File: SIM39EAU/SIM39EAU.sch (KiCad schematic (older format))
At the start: 15 parts, among them IC1 SIM39EA, J1 Conn_01x08, U2 AP7365-W-7

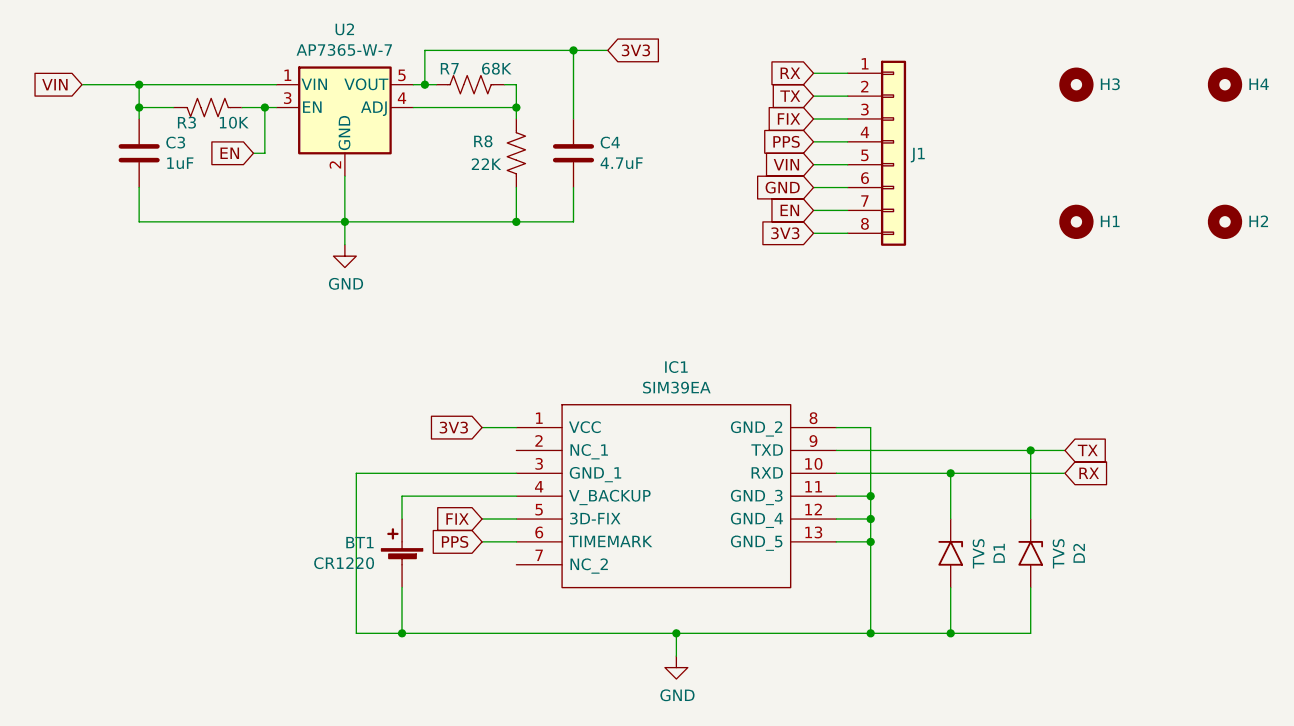
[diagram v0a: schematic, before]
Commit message: LED Update
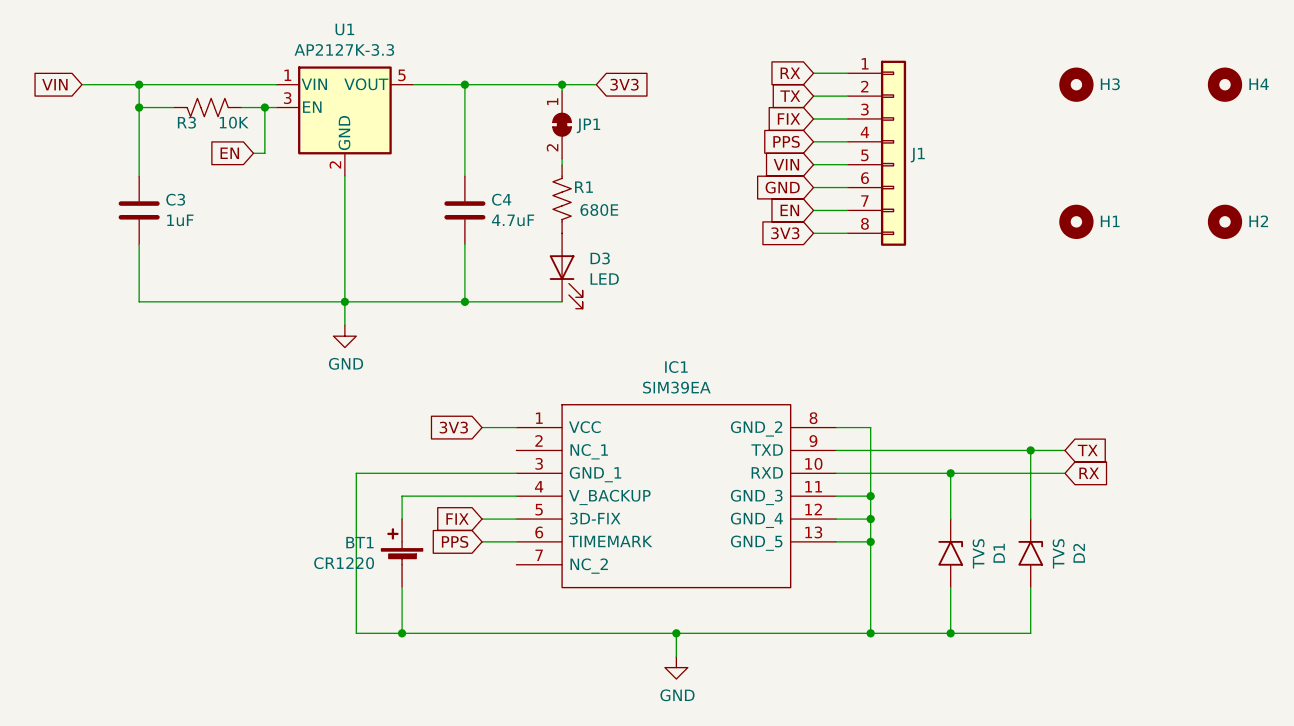
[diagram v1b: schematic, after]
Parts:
- removed R7: 68K, Resistor_SMD:R_0603_1608Metric, symbol Device:R_US
- removed R8: 22K, Resistor_SMD:R_0603_1608Metric, symbol Device:R_US
- removed U2: AP7365-W-7, Package_TO_SOT_SMD:SOT-23-5, symbol Regulator_Linear:AP2127K-ADJ
- added D3: LED, LED_SMD:LED_0603_1608Metric, symbol Device:LED
- added JP1: SolderJumper_2_Bridged, Jumper:SolderJumper-2_P1.3mm_Bridged_RoundedPad1.0x1.5mm, symbol Jumper:SolderJumper_2_Bridged
- added R1: 680E, Resistor_SMD:R_0603_1608Metric, symbol Device:R_US
- added U1: AP2127K-3.3, Package_TO_SOT_SMD:SOT-23-5, symbol Regulator_Linear:AP2127K-3.3
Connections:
- net 3V3: now also JP1.1 (A), U1.5 (VOUT)
- net EN: now also U1.3 (EN)
- net GND: now also D3.1 (K), U1.2 (GND)
- net VIN: now also U1.1 (VIN)
- new net: JP1.2 (B), R1.2
- new net: D3.2 (A), R1.1
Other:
- moved on the sheet: C3, C4
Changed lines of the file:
@@
 Comment4 ""
 $EndDescr
-Text GLabel 3600 1100 2    50   Input ~ 0
+Text GLabel 3550 1250 2    50   Input ~ 0
 3V3
 Wire Wire Line
-	1550 1400 1550 1350
-Wire Wire Line
-	1550 1700 1550 1850
+	1550 1650 1550 1350
+Wire Wire Line
+	1550 1950 1550 2200
 $Comp
 L power:GND #PWR0103
 U 1 1 5DFA7870
-P 2450 1950
-F 0 "#PWR0103" H 2450 1700 50  0001 C CNN
-F 1 "GND" H 2455 1777 50  0000 C CNN
-F 2 "" H 2450 1950 50  0001 C CNN
-F 3 "" H 2450 1950 50  0001 C CNN
-	1    2450 1950
-	1    0    0    -1
-$EndComp
-$Comp
-L Regulator_Linear:AP2127K-ADJ U2
-U 1 1 5E2BA0AD
-P 2450 1350
-F 0 "U2" H 2450 1690 50  0000 C CNN
-F 1 "AP7365-W-7" H 2450 1600 50  0000 C CNN
-F 2 "Package_TO_SOT_SMD:SOT-23-5" H 2450 1675 50  0001 C CNN
-F 3 "https://www.diodes.com/assets/Datasheets/AP2127.pdf" H 2450 1450 50  0001 C CNN
-	1    2450 1350
-	1    0    0    -1
-$EndComp
-$Comp
-L Device:R_US R7
-U 1 1 5E34715F
-P 3000 1250
-F 0 "R7" V 3068 1296 50  0000 L CNN
-F 1 "68K" V 3068 1205 50  0000 R CNN
-F 2 "Resistor_SMD:R_0603_1608Metric" V 3040 1240 50  0001 C CNN
-F 3 "~" H 3000 1250 50  0001 C CNN
-F 4 "C163436" V 3000 1250 50  0001 C CNN "Part"
-	1    3000 1250
-	0    -1   -1   0
-$EndComp
-$Comp
-L Device:R_US R8
-U 1 1 5E35753D
-P 3200 1550
-F 0 "R8" H 3300 1500 50  0000 L CNN
-F 1 "22K" H 3400 1600 50  0000 R CNN
-F 2 "Resistor_SMD:R_0603_1608Metric" V 3240 1540 50  0001 C CNN
-F 3 "~" H 3200 1550 50  0001 C CNN
-F 4 "C103426" H 3200 1550 50  0001 C CNN "Part"
-	1    3200 1550
-	-1   0    0    1
-$EndComp
-Wire Wire Line
-	3200 1350 2750 1350
-Wire Wire Line
-	3150 1250 3200 1250
-Wire Wire Line
-	3200 1400 3200 1350
+P 2450 2300
+F 0 "#PWR0103" H 2450 2050 50  0001 C CNN
+F 1 "GND" H 2455 2127 50  0000 C CNN
+F 2 "" H 2450 2300 50  0001 C CNN
+F 3 "" H 2450 2300 50  0001 C CNN
+	1    2450 2300
+	1    0    0    -1
+$EndComp
 Text GLabel 4500 1300 0    50   Input ~ 0
 TX
@@
 FIX
 Wire Wire Line
-	1550 1850 2450 1850
-Wire Wire Line
-	3200 1700 3200 1850
-Wire Wire Line
-	3200 1350 3200 1250
-Connection ~ 3200 1350
-Wire Wire Line
-	2750 1250 2800 1250
-Wire Wire Line
-	2800 1250 2800 1100
-Connection ~ 2800 1250
-Wire Wire Line
-	2800 1250 2850 1250
-Wire Wire Line
-	2800 1100 3450 1100
+	1550 2200 2450 2200
 $Comp
 L Device:C C3
 U 1 1 5DCB3070
-P 1550 1550
-F 0 "C3" H 1665 1595 50  0000 L CNN
-F 1 "1uF" H 1665 1505 50  0000 L CNN
-F 2 "Capacitor_SMD:C_0805_2012Metric" H 1588 1400 50  0001 C CNN
-F 3 "~" H 1550 1550 50  0001 C CNN
-F 4 "C396719" H 1550 1550 50  0001 C CNN "Part"
-	1    1550 1550
-	1    0    0    -1
-$EndComp
-Wire Wire Line
-	3450 1400 3450 1100
-Connection ~ 3450 1100
-Wire Wire Line
-	3450 1100 3600 1100
-Wire Wire Line
-	3450 1700 3450 1850
-Wire Wire Line
-	3450 1850 3200 1850
-Connection ~ 3200 1850
+P 1550 1800
+F 0 "C3" H 1665 1845 50  0000 L CNN
+F 1 "1uF" H 1665 1755 50  0000 L CNN
+F 2 "Capacitor_SMD:C_0805_2012Metric" H 1588 1650 50  0001 C CNN
+F 3 "~" H 1550 1800 50  0001 C CNN
+F 4 "C396719" H 1550 1800 50  0001 C CNN "Part"
+	1    1550 1800
+	1    0    0    -1
+$EndComp
+Wire Wire Line
+	2975 1950 2975 2200
 Text GLabel 1300 1250 0    50   Input ~ 0
 VIN
@@
 L Device:C C4
 U 1 1 5DB8E885
-P 3450 1550
-F 0 "C4" H 3565 1595 50  0000 L CNN
-F 1 "4.7uF" H 3565 1505 50  0000 L CNN
-F 2 "Capacitor_SMD:C_0805_2012Metric" H 3488 1400 50  0001 C CNN
-F 3 "~" H 3450 1550 50  0001 C CNN
-F 4 "C87998" H 3450 1550 50  0001 C CNN "Part"
-	1    3450 1550
+P 2975 1800
+F 0 "C4" H 3090 1845 50  0000 L CNN
+F 1 "4.7uF" H 3090 1755 50  0000 L CNN
+F 2 "Capacitor_SMD:C_0805_2012Metric" H 3013 1650 50  0001 C CNN
+F 3 "~" H 2975 1800 50  0001 C CNN
+F 4 "C87998" H 2975 1800 50  0001 C CNN "Part"
+	1    2975 1800
 	1    0    0    -1
 $EndComp
@@
 	1    0    0    -1
 $EndComp
-Wire Wire Line
-	2450 1650 2450 1850
-Connection ~ 2450 1850
-Wire Wire Line
-	2450 1850 3200 1850
-Wire Wire Line
-	2450 1850 2450 1950
+Connection ~ 2450 2200
+Wire Wire Line
+	2450 2200 2450 2300
 Wire Wire Line
 	4650 1500 4500 1500
@@
 Wire Wire Line
 	5100 3450 5100 3650
+Wire Wire Line
+	2450 2200 2975 2200
+Wire Wire Line
+	2750 1250 2975 1250
+$Comp
+L Regulator_Linear:AP2127K-3.3 U1
+U 1 1 5DFE50D8
+P 2450 1350
+F 0 "U1" H 2450 1690 50  0000 C CNN
+F 1 "AP2127K-3.3" H 2450 1600 50  0000 C CNN
+F 2 "Package_TO_SOT_SMD:SOT-23-5" H 2450 1675 50  0001 C CNN
+F 3 "https://www.diodes.com/assets/Datasheets/AP2127.pdf" H 2450 1450 50  0001 C CNN
+	1    2450 1350
+	1    0    0    -1
+$EndComp
+Wire Wire Line
+	2975 1650 2975 1250
+Wire Wire Line
+	2450 1650 2450 2200
+Connection ~ 2975 1250
+Connection ~ 2975 2200
+Wire Wire Line
+	2975 1250 3400 1250
+$Comp
+L Jumper:SolderJumper_2_Bridged JP1
+U 1 1 5DFFCA44
+P 3400 1425
+F 0 "JP1" V 3400 1493 50  0000 L CNN
+F 1 "SolderJumper_2_Bridged" V 3445 1493 50  0001 L CNN
+F 2 "Jumper:SolderJumper-2_P1.3mm_Bridged_RoundedPad1.0x1.5mm" H 3400 1425 50  0001 C CNN
+F 3 "~" H 3400 1425 50  0001 C CNN
+	1    3400 1425
+	0    1    1    0
+$EndComp
+$Comp
+L Device:LED D3
+U 1 1 5DFFF072
+P 3400 2050
+F 0 "D3" V 3438 1932 50  0000 R CNN
+F 1 "LED" V 3348 1932 50  0000 R CNN
+F 2 "LED_SMD:LED_0603_1608Metric" H 3400 2050 50  0001 C CNN
+F 3 "~" H 3400 2050 50  0001 C CNN
+F 4 "C193191" V 3400 2050 50  0001 C CNN "Part"
+	1    3400 2050
+	0    -1   -1   0
+$EndComp
+$Comp
+L Device:R_US R1
+U 1 1 5E000844
+P 3400 1750
+F 0 "R1" H 3450 1700 50  0000 L CNN
+F 1 "680E" H 3650 1800 50  0000 R CNN
+F 2 "Resistor_SMD:R_0603_1608Metric" V 3440 1740 50  0001 C CNN
+F 3 "~" H 3400 1750 50  0001 C CNN
+F 4 "C269441" V 3400 1750 50  0001 C CNN "Part"
+	1    3400 1750
+	1    0    0    1
+$EndComp
+Wire Wire Line
+	2975 2200 3400 2200
+Wire Wire Line
+	3400 1600 3400 1575
+Wire Wire Line
+	3400 1275 3400 1250
+Connection ~ 3400 1250
+Wire Wire Line
+	3400 1250 3550 1250
 $EndSCHEMATC

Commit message: Schematic PDF and 3D Renders added
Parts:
- IC1: symbol SIM39EA:SIM39EA -> SIM39EAU-rescue:SIM39EA-SIM39EA
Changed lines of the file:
@@
 	4650 1600 4500 1600
 $Comp
-L SIM39EA:SIM39EA IC1
+L SIM39EAU-rescue:SIM39EA-SIM39EA IC1
 U 1 1 5DC20384
 P 3200 2750
